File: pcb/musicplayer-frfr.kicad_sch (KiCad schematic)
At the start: 22 parts, among them J1 Battery, J2 AudioPlug3, J3 Display, SW1 SW_Push, SW2 SW_Push, SW3 SW_Push, SW4 RotaryEncoder_Switch, U1 XIAO-RP2350-SMD, U2 TP4056-42-ESOP8, U3 DFPLAYER_MINI

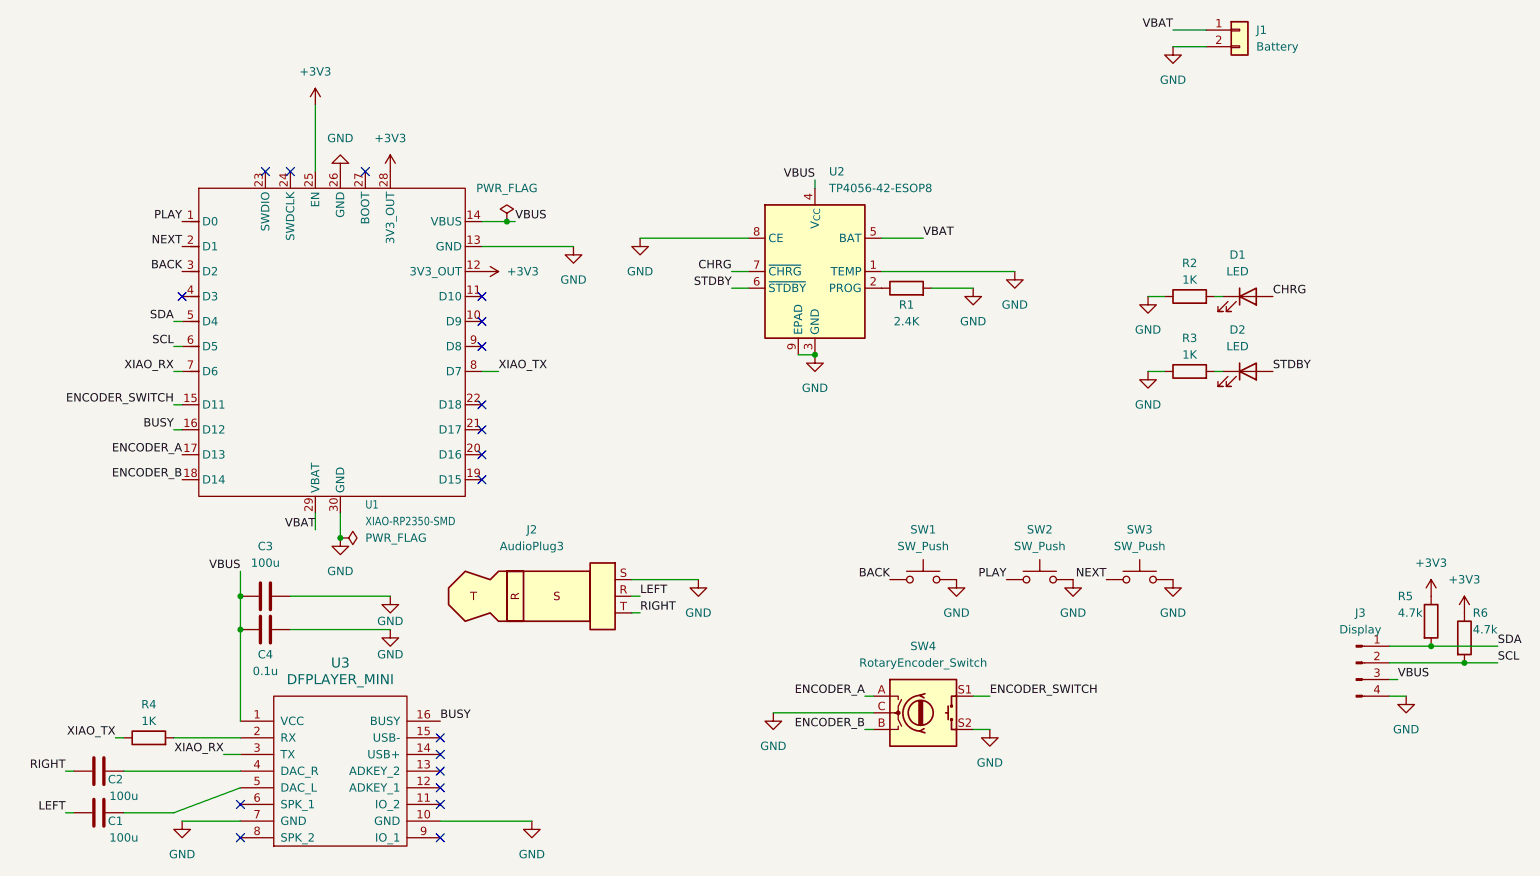
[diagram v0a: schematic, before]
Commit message: fix up pcb with cool new rounded corners and some layout changes. also added a power switch
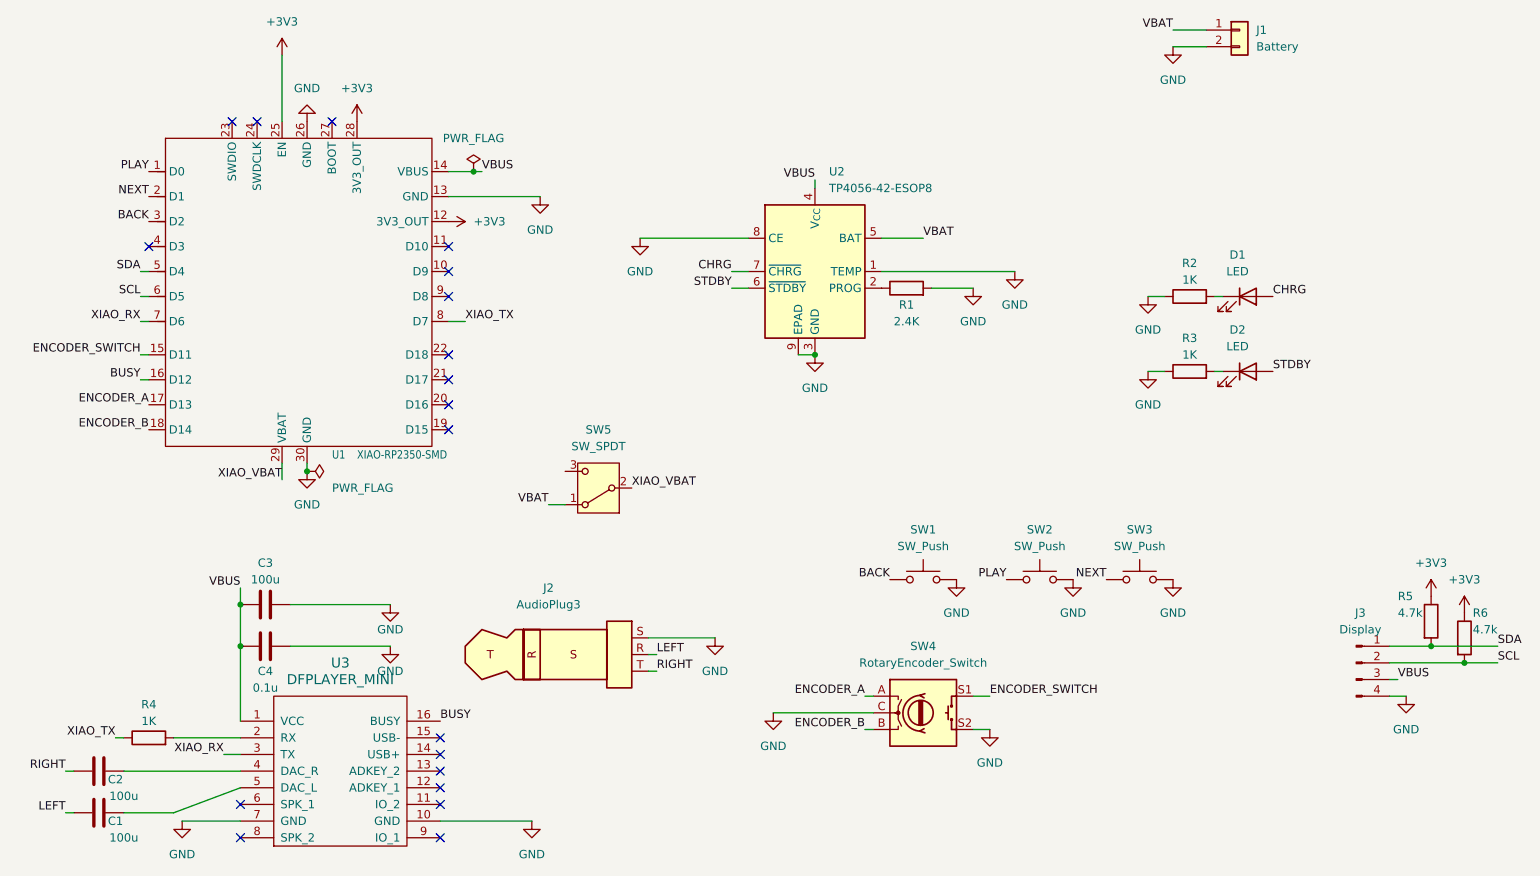
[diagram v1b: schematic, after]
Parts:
- added SW5: SW_SPDT, Button_Switch_THT:SW_Slide_SPDT_Straight_CK_OS102011MS2Q, symbol Switch:SW_SPDT
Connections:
- net VBAT: now also SW5.1 (A); no longer U1.29 (VBAT)
- new net XIAO_VBAT: SW5.2 (B), U1.29 (VBAT)
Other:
- moved on the sheet: C3, C4, J2, U1
